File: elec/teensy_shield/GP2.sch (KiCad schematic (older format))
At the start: 1 part

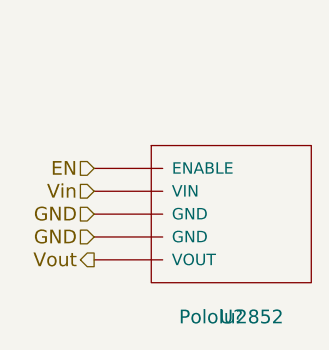
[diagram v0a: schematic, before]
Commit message: Completed new board schematics.
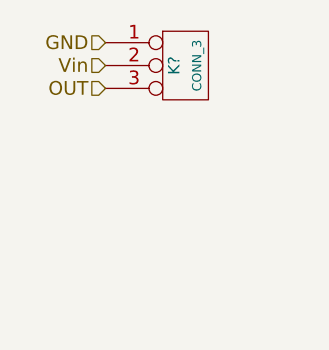
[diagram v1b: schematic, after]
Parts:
- removed U?: Pololu2852, symbol Pololu2852
- added K?: CONN_3, symbol CONN_3
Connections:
- net GND: now also K?.1 (P1)
- net Vin: now also K?.2 (PM)
- new net OUT: K?.3 (P3)
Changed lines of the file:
@@
 $Descr A4 11693 8268
 encoding utf-8
-Sheet 9 34
+Sheet 34 34
 Title ""
 Date ""
@@
 Comment4 ""
 $EndDescr
-Text HLabel 5200 3950 0    60   Input ~ 0
+Text HLabel 5250 3100 0    60   Input ~ 0
 GND
-Text HLabel 5200 3750 0    60   Input ~ 0
+Text HLabel 5250 3200 0    60   Input ~ 0
 Vin
-Text HLabel 5200 4050 0    60   Output ~ 0
-Vout
-Text HLabel 5200 3650 0    60   Input ~ 0
-EN
+Text HLabel 5250 3300 0    60   Input ~ 0
+OUT
 $Comp
-L Pololu2852 U?
-U 1 1 55E8368A
-P 5850 3900
-F 0 "U?" H 5800 3500 60  0000 C CNN
-F 1 "Pololu2852" H 5800 3500 60  0000 C CNN
-F 2 "" H 5800 3500 60  0000 C CNN
-F 3 "" H 5800 3500 60  0000 C CNN
-	1    5850 3900
+L CONN_3 K?
+U 1 1 55E84D77
+P 5600 3200
+F 0 "K?" V 5550 3200 50  0000 C CNN
+F 1 "CONN_3" V 5650 3200 40  0000 C CNN
+F 2 "" H 5600 3200 60  0000 C CNN
+F 3 "" H 5600 3200 60  0000 C CNN
+	1    5600 3200
 	1    0    0    -1
 $EndComp
-Text HLabel 5200 3850 0    60   Input ~ 0
-GND
 $EndSCHEMATC
